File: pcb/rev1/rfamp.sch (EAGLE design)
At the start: 17 parts, among them IC1 TS520530, IC2 ADL5523, X1 SAW-B3721

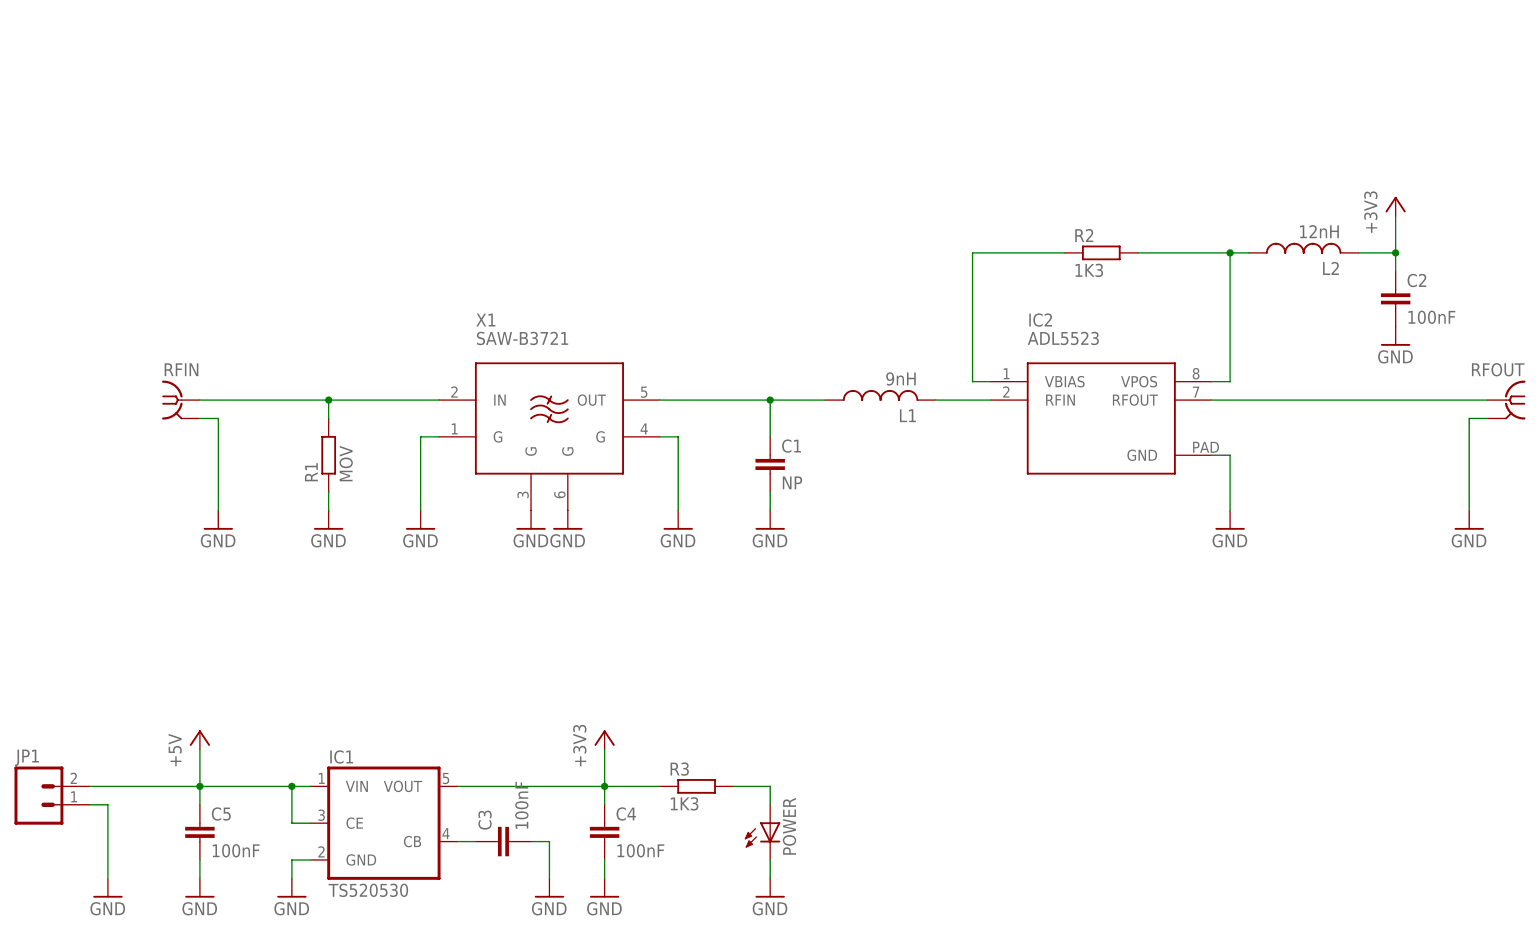
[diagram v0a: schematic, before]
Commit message: Minor changes.
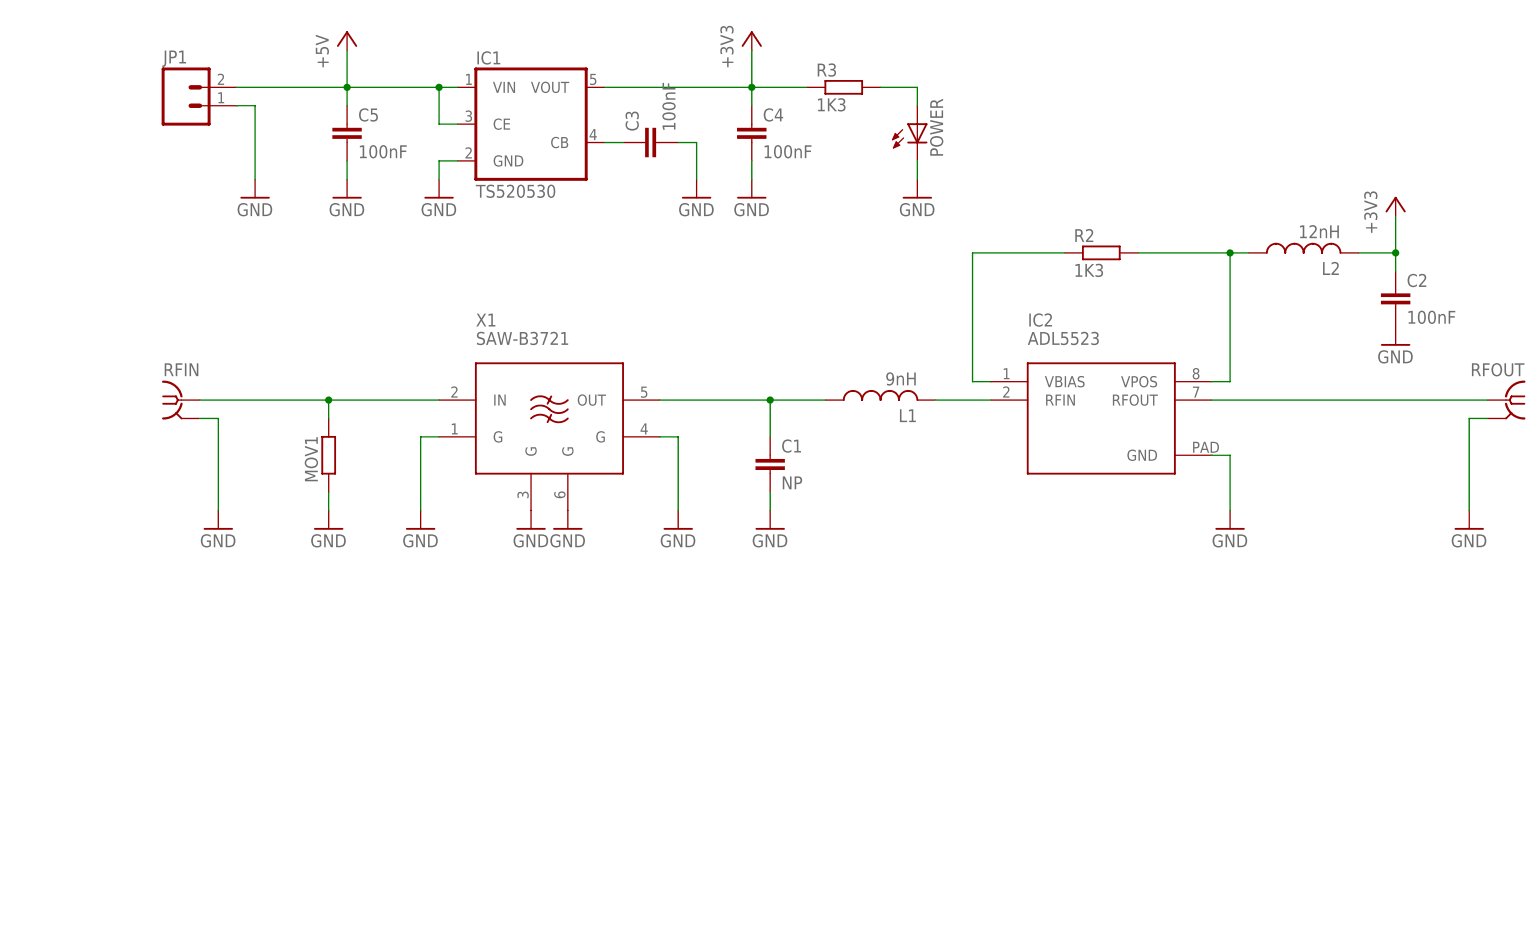
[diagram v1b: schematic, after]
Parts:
- MOV1: value MOV -> (none)
- renumbered R1 to MOV1
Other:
- moved on the sheet: C3, C4, C5, IC1, JP1, POWER, R3
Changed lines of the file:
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@@
 <part name="GND3" library="supply1" deviceset="GND" device=""/>
 <part name="X1" library="qyx-misc" deviceset="SAW-B3721" device=""/>
-<part name="R1" library="rcl" deviceset="R-EU_" device="R0603" value="MOV"/>
+<part name="MOV1" library="rcl" deviceset="R-EU_" device="R0603"/>
 <part name="GND4" library="supply1" deviceset="GND" device=""/>
 <part name="GND5" library="supply1" deviceset="GND" device=""/>
@@
 <instance part="RFIN" gate="G1" x="0" y="71.12"/>
 <instance part="GND1" gate="1" x="5.08" y="53.34"/>
-<instance part="GND2" gate="1" x="2.54" y="2.54"/>
+<instance part="GND2" gate="1" x="22.86" y="99.06"/>
 <instance part="RFOUT" gate="G1" x="182.88" y="71.12" rot="MR0"/>
 <instance part="GND3" gate="1" x="177.8" y="53.34"/>
 <instance part="X1" gate="G$1" x="53.34" y="66.04"/>
-<instance part="R1" gate="G$1" x="20.32" y="63.5" rot="R90"/>
+<instance part="MOV1" gate="G$1" x="20.32" y="63.5" rot="R90"/>
 <instance part="GND4" gate="1" x="48.26" y="53.34"/>
 <instance part="GND5" gate="1" x="53.34" y="53.34"/>
@@
 <instance part="GND10" gate="1" x="167.64" y="78.74"/>
 <instance part="+3V1" gate="G$1" x="167.64" y="99.06"/>
-<instance part="+3V2" gate="G$1" x="58.42" y="25.4"/>
-<instance part="IC1" gate="G$1" x="27.94" y="12.7"/>
-<instance part="C3" gate="G$1" x="43.18" y="10.16" rot="R90"/>
-<instance part="C4" gate="G$1" x="58.42" y="12.7"/>
-<instance part="C5" gate="G$1" x="2.54" y="12.7"/>
-<instance part="GND11" gate="1" x="15.24" y="2.54"/>
-<instance part="GND12" gate="1" x="50.8" y="2.54"/>
-<instance part="GND13" gate="1" x="58.42" y="2.54"/>
-<instance part="P+1" gate="1" x="2.54" y="25.4"/>
-<instance part="JP1" gate="G$1" x="-20.32" y="15.24"/>
-<instance part="GND14" gate="1" x="-10.16" y="2.54"/>
+<instance part="+3V2" gate="G$1" x="78.74" y="121.92"/>
+<instance part="IC1" gate="G$1" x="48.26" y="109.22"/>
+<instance part="C3" gate="G$1" x="63.5" y="106.68" rot="R90"/>
+<instance part="C4" gate="G$1" x="78.74" y="109.22"/>
+<instance part="C5" gate="G$1" x="22.86" y="109.22"/>
+<instance part="GND11" gate="1" x="35.56" y="99.06"/>
+<instance part="GND12" gate="1" x="71.12" y="99.06"/>
+<instance part="GND13" gate="1" x="78.74" y="99.06"/>
+<instance part="P+1" gate="1" x="22.86" y="121.92"/>
+<instance part="JP1" gate="G$1" x="0" y="111.76"/>
+<instance part="GND14" gate="1" x="10.16" y="99.06"/>
 <instance part="IC2" gate="G$1" x="127" y="68.58"/>
 <instance part="GND15" gate="1" x="144.78" y="53.34"/>
-<instance part="R3" gate="G$1" x="71.12" y="17.78"/>
-<instance part="POWER" gate="G$1" x="81.28" y="12.7"/>
-<instance part="GND16" gate="1" x="81.28" y="2.54"/>
+<instance part="R3" gate="G$1" x="91.44" y="114.3"/>
+<instance part="POWER" gate="G$1" x="101.6" y="109.22"/>
+<instance part="GND16" gate="1" x="101.6" y="99.06"/>
 </instances>
 <busses>
@@
 <segment>
 <pinref part="GND8" gate="1" pin="GND"/>
-<pinref part="R1" gate="G$1" pin="1"/>
+<pinref part="MOV1" gate="G$1" pin="1"/>
 <wire x1="20.32" y1="55.88" x2="20.32" y2="58.42" width="0.1524" layer="91"/>
 </segment>
@@
 <pinref part="C5" gate="G$1" pin="2"/>
 <pinref part="GND2" gate="1" pin="GND"/>
-<wire x1="2.54" y1="7.62" x2="2.54" y2="5.08" width="0.1524" layer="91"/>
+<wire x1="22.86" y1="104.14" x2="22.86" y2="101.6" width="0.1524" layer="91"/>
 </segment>
 <segment>
 <pinref part="IC1" gate="G$1" pin="GND"/>
 <pinref part="GND11" gate="1" pin="GND"/>
-<wire x1="17.78" y1="7.62" x2="15.24" y2="7.62" width="0.1524" layer="91"/>
-<wire x1="15.24" y1="7.62" x2="15.24" y2="5.08" width="0.1524" layer="91"/>
+<wire x1="38.1" y1="104.14" x2="35.56" y2="104.14" width="0.1524" layer="91"/>
+<wire x1="35.56" y1="104.14" x2="35.56" y2="101.6" width="0.1524" layer="91"/>
 </segment>
 <segment>
 <pinref part="C4" gate="G$1" pin="2"/>
 <pinref part="GND13" gate="1" pin="GND"/>
-<wire x1="58.42" y1="7.62" x2="58.42" y2="5.08" width="0.1524" layer="91"/>
+<wire x1="78.74" y1="104.14" x2="78.74" y2="101.6" width="0.1524" layer="91"/>
 </segment>
 <segment>
 <pinref part="C3" gate="G$1" pin="2"/>
 <pinref part="GND12" gate="1" pin="GND"/>
-<wire x1="48.26" y1="10.16" x2="50.8" y2="10.16" width="0.1524" layer="91"/>
-<wire x1="50.8" y1="10.16" x2="50.8" y2="5.08" width="0.1524" layer="91"/>
+<wire x1="68.58" y1="106.68" x2="71.12" y2="106.68" width="0.1524" layer="91"/>
+<wire x1="71.12" y1="106.68" x2="71.12" y2="101.6" width="0.1524" layer="91"/>
 </segment>
 <segment>
 <pinref part="JP1" gate="G$1" pin="1"/>
 <pinref part="GND14" gate="1" pin="GND"/>
-<wire x1="-12.7" y1="15.24" x2="-10.16" y2="15.24" width="0.1524" layer="91"/>
-<wire x1="-10.16" y1="15.24" x2="-10.16" y2="5.08" width="0.1524" layer="91"/>
+<wire x1="7.62" y1="111.76" x2="10.16" y2="111.76" width="0.1524" layer="91"/>
+<wire x1="10.16" y1="111.76" x2="10.16" y2="101.6" width="0.1524" layer="91"/>
 </segment>
 <segment>
@@
 <pinref part="POWER" gate="G$1" pin="C"/>
 <pinref part="GND16" gate="1" pin="GND"/>
-<wire x1="81.28" y1="7.62" x2="81.28" y2="5.08" width="0.1524" layer="91"/>
+<wire x1="101.6" y1="104.14" x2="101.6" y2="101.6" width="0.1524" layer="91"/>
 </segment>
 </net>
@@
 <segment>
 <pinref part="RFIN" gate="G1" pin="1"/>
-<pinref part="R1" gate="G$1" pin="2"/>
+<pinref part="MOV1" gate="G$1" pin="2"/>
 <wire x1="2.54" y1="71.12" x2="20.32" y2="71.12" width="0.1524" layer="91"/>
 <wire x1="20.32" y1="71.12" x2="20.32" y2="68.58" width="0.1524" layer="91"/>
@@
 <pinref part="IC1" gate="G$1" pin="VOUT"/>
 <pinref part="C4" gate="G$1" pin="1"/>
-<wire x1="38.1" y1="17.78" x2="58.42" y2="17.78" width="0.1524" layer="91"/>
-<wire x1="58.42" y1="17.78" x2="58.42" y2="15.24" width="0.1524" layer="91"/>
+<wire x1="58.42" y1="114.3" x2="78.74" y2="114.3" width="0.1524" layer="91"/>
+<wire x1="78.74" y1="114.3" x2="78.74" y2="111.76" width="0.1524" layer="91"/>
 <pinref part="+3V2" gate="G$1" pin="+3V3"/>
-<wire x1="58.42" y1="17.78" x2="58.42" y2="22.86" width="0.1524" layer="91"/>
-<junction x="58.42" y="17.78"/>
+<wire x1="78.74" y1="114.3" x2="78.74" y2="119.38" width="0.1524" layer="91"/>
+<junction x="78.74" y="114.3"/>
 <pinref part="R3" gate="G$1" pin="1"/>
-<wire x1="58.42" y1="17.78" x2="66.04" y2="17.78" width="0.1524" layer="91"/>
+<wire x1="78.74" y1="114.3" x2="86.36" y2="114.3" width="0.1524" layer="91"/>
 </segment>
 </net>
@@
 <pinref part="C5" gate="G$1" pin="1"/>
 <pinref part="P+1" gate="1" pin="+5V"/>
-<wire x1="2.54" y1="15.24" x2="2.54" y2="17.78" width="0.1524" layer="91"/>
+<wire x1="22.86" y1="111.76" x2="22.86" y2="114.3" width="0.1524" layer="91"/>
 <pinref part="IC1" gate="G$1" pin="VIN"/>
-<wire x1="2.54" y1="17.78" x2="2.54" y2="22.86" width="0.1524" layer="91"/>
-<wire x1="17.78" y1="17.78" x2="15.24" y2="17.78" width="0.1524" layer="91"/>
-<junction x="2.54" y="17.78"/>
+<wire x1="22.86" y1="114.3" x2="22.86" y2="119.38" width="0.1524" layer="91"/>
+<wire x1="38.1" y1="114.3" x2="35.56" y2="114.3" width="0.1524" layer="91"/>
+<junction x="22.86" y="114.3"/>
 <pinref part="IC1" gate="G$1" pin="CE"/>
-<wire x1="15.24" y1="17.78" x2="2.54" y2="17.78" width="0.1524" layer="91"/>
-<wire x1="17.78" y1="12.7" x2="15.24" y2="12.7" width="0.1524" layer="91"/>
-<wire x1="15.24" y1="12.7" x2="15.24" y2="17.78" width="0.1524" layer="91"/>
-<junction x="15.24" y="17.78"/>
+<wire x1="35.56" y1="114.3" x2="22.86" y2="114.3" width="0.1524" layer="91"/>
+<wire x1="38.1" y1="109.22" x2="35.56" y2="109.22" width="0.1524" layer="91"/>
+<wire x1="35.56" y1="109.22" x2="35.56" y2="114.3" width="0.1524" layer="91"/>
+<junction x="35.56" y="114.3"/>
 <pinref part="JP1" gate="G$1" pin="2"/>
-<wire x1="-12.7" y1="17.78" x2="2.54" y2="17.78" width="0.1524" layer="91"/>
+<wire x1="7.62" y1="114.3" x2="22.86" y2="114.3" width="0.1524" layer="91"/>
 </segment>
 </net>
@@
 <pinref part="C3" gate="G$1" pin="1"/>
 <pinref part="IC1" gate="G$1" pin="CB"/>
-<wire x1="40.64" y1="10.16" x2="38.1" y2="10.16" width="0.1524" layer="91"/>
+<wire x1="60.96" y1="106.68" x2="58.42" y2="106.68" width="0.1524" layer="91"/>
 </segment>
 </net>
@@
 <pinref part="R3" gate="G$1" pin="2"/>
 <pinref part="POWER" gate="G$1" pin="A"/>
-<wire x1="76.2" y1="17.78" x2="81.28" y2="17.78" width="0.1524" layer="91"/>
-<wire x1="81.28" y1="17.78" x2="81.28" y2="15.24" width="0.1524" layer="91"/>
-</segment>
-</net>
+<wire x1="96.52" y1="114.3" x2="101.6" y2="114.3" width="0.1524" layer="91"/>
+<wire x1="101.6" y1="114.3" x2="101.6" y2="111.76" width="0.1524" layer="91"/>
+</segment>
+</net>
